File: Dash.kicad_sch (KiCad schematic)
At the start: 159 parts, among them J10 Conn_01x04_Socket, J11 Conn_01x04_Socket, J12 Conn_01x06_Socket, J13 Conn_01x06_Socket, J14 Conn_01x06_Socket, J15 Conn_01x06_Socket, J2 Conn_01x06_Socket, J4 Conn_01x03_Socket, J5 Conn_01x04_Socket, J6 Conn_01x04_Socket, J7 Conn_01x04_Socket, J8 Conn_01x04_Socket, J9 Conn_01x04_Socket, Q1 NPN, Q10 NPN, Q11 NPN, Q12 NPN, Q13 NPN, Q14 NPN, Q15 NPN, Q16 NPN, Q17 NPN, Q18 NPN, Q19 PMOS, Q2 NPN, Q20 NMOS, Q21 NPN, Q3 NPN, Q4 NPN, Q5 NPN, Q6 NPN, Q7 NPN, Q8 NPN, Q9 NPN, SW1 SW_Push, U1 LM2678T-5.0, U10 L293D, U11 L293D, U12 L293D, U13 L293D, U14 L293D, U15 L293D, U16 SFH617A-1, U2 ADS1015IDGS, U4 24C02Cx-x-SN, U5 ESP32-S2-DevKitM, U6 24C02Cx-x-SN, U7 74HC595, U8 74HC595, U9 74HC595

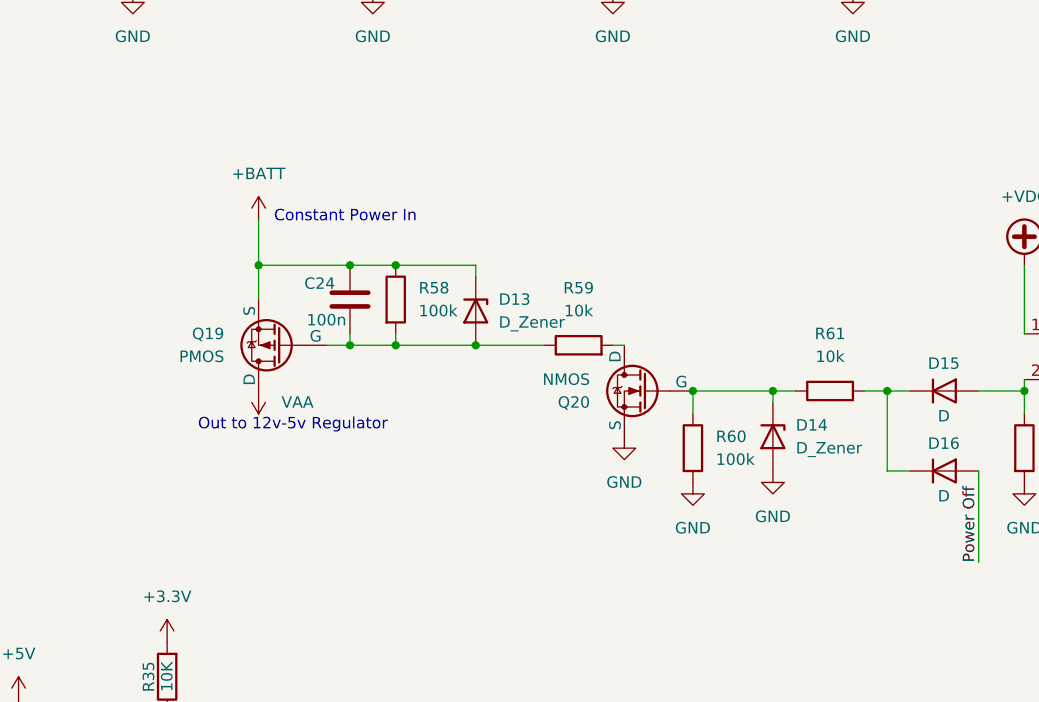
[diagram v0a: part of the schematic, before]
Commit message: update power latch
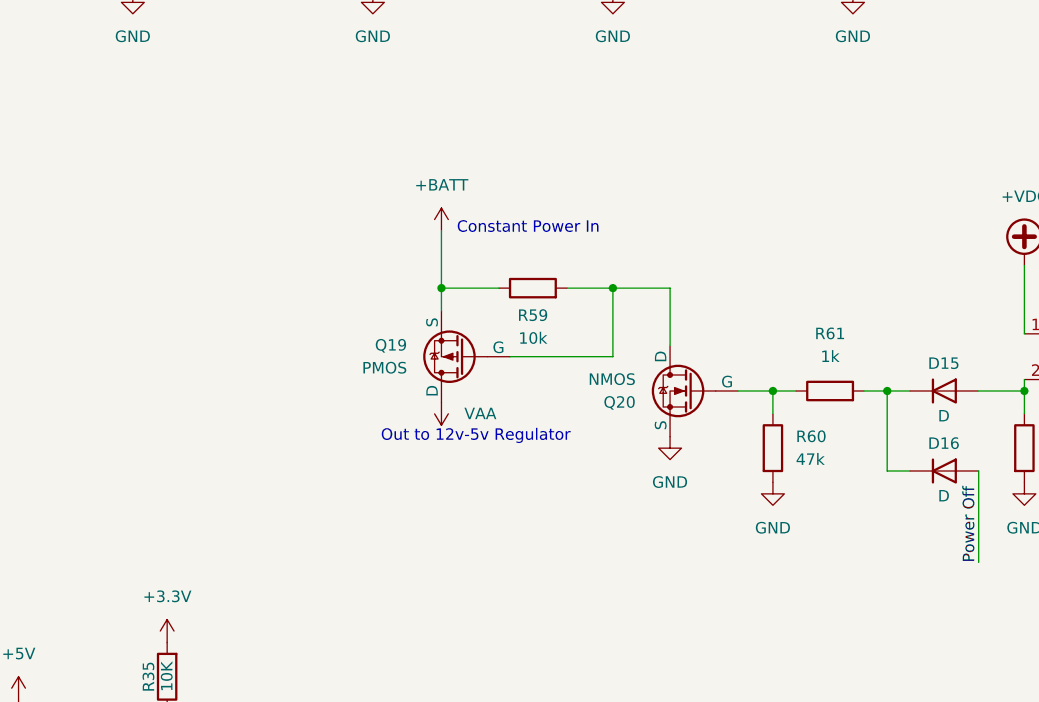
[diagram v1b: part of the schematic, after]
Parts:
- removed C24: 100n, symbol Device:C
- removed D13, D14: D_Zener, symbol Device:D_Zener
- removed R58: 100k, symbol Device:R
- R60: value 100k -> 47k
- R61: value 10k -> 1k
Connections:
- net +BATT: now also R59.1
- net at Q19.2 (G): now also Q20.1 (D), R59.2; no longer R59.1
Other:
- moved on the sheet: Q19, Q20, R59, R60
